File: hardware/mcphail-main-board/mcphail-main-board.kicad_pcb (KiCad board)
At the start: 2 copper layers, 80.6 x 56.6 mm, 143 parts, among them J1 INSECT DETECTION, J2 EMITTERS, J3 BREAKOUT, J4 MICRO SD, J5 MICRO USB, J6 PROG/BOOT, J7 FONA 808, J8 INPUT 6V-9V, J9 JST PH, U1 MCP6004, U10 BUCK-BOOST 5V TPS63060, U11 MCP1703, U2 MCP6004, U3 TLV274, U4 MCP6001, U5 ADS1118, U6 ATSAMD21G18A, U7 24AA1025 EEPROM, U8 MCP7940N RTC, U9 MCP73871, X1 16MHz, X2 32.768kHz

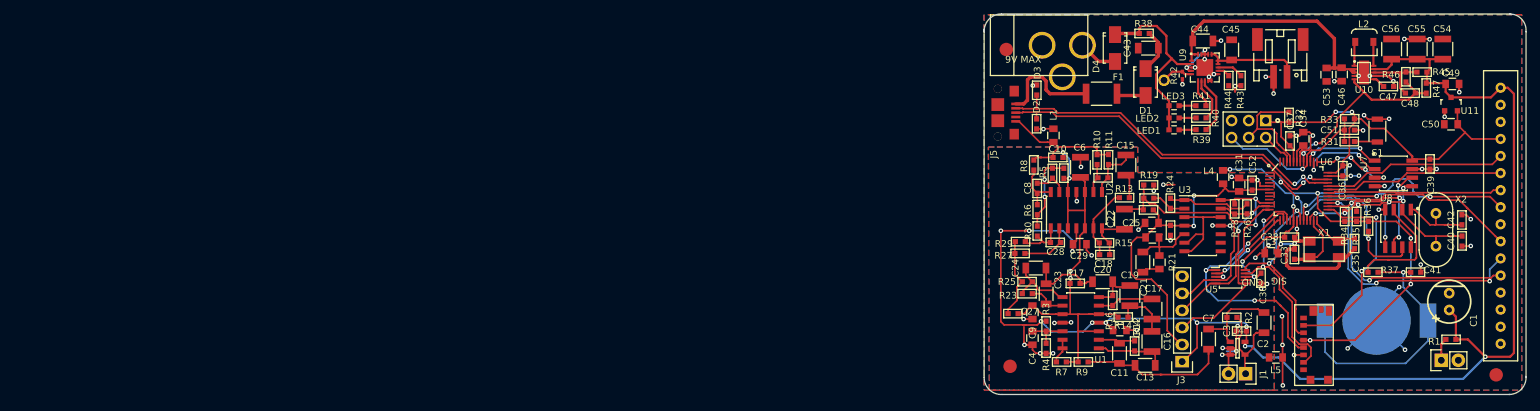
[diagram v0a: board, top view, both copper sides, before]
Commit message: Release v1.0 McPhail Main Board
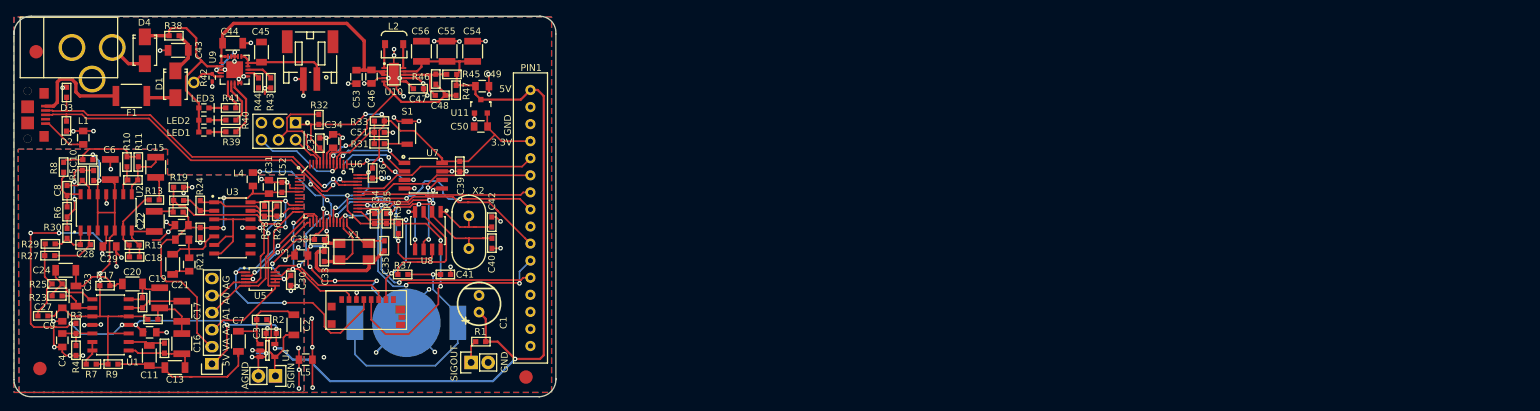
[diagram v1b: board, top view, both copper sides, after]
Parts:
- moved BAT1 144.4 mm to (81.7, 87.8)
- moved C1 144.4 mm to (92.5, 84.9)
- moved C10 144.4 mm to (34.3, 63.5)
- moved C11 144.4 mm to (43.4, 92.6)
- moved C12 144.4 mm to (40.9, 66.5)
- moved C13 144.4 mm to (47.2, 94.4)
- moved C14 144.4 mm to (43.5, 89.2)
- moved C15 144.4 mm to (44.4, 64.6)
- moved C16 144.4 mm to (48.2, 90.9)
- moved C17 144.4 mm to (48.2, 86.0)
- moved C2 144.4 mm to (64.9, 88.1)
- moved C20 144.4 mm to (40.9, 82.0)
- moved C21 144.4 mm to (46.9, 79.1)
- moved C22 144.4 mm to (44.1, 72.7)
- moved C23 144.4 mm to (32.5, 83.8)
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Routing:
- net GND: track 127.3 -> 171.4 mm, vias 45 -> 57
- net AGND: track 52.7 -> 67.3 mm, vias 26 -> 32
- net /Microcontroller/D7_CS: track 30.8 -> 21.0 mm
- net /Microcontroller/MISO: track 34.3 -> 25.8 mm
- net +3V3: track 156.4 -> 150.2 mm, vias 11 -> 10
- net /Microcontroller/SCLK: track 40.6 -> 45.8 mm
- net /Microcontroller/MOSI: track 28.4 -> 30.1 mm
- net (no net): track 1.71 -> 0.00 mm
- net /Microcontroller/SDA: track 28.5 -> 29.2 mm
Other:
- board text added: "3.3V"
- board text added: "5V"
- board text added: "5V VA A2 A1 A0 AG"
- board text added: "AGND"
- board text added: "FABRICATION NOTES 1. THIS IS A 2 LAYER BOARD. 2. EXTERNAL LAYERS SHALL HAVE 1 OZ COPPER. 3. MATERIAL: FR4 AND 0.062 INCH +/- 10% THICK. 4. BOARDS SHALL BE ROHS COMPLIANT. 5. MANUFACTURE IN ACCORDANCE WITH IPC-6012 CLASS 2 6. MASK: BOTH SIDES OF THE BOARD SHALL HAVE SOLDER MASK (ANY COLOR) OVER BARE COPPER. 7. SILK: BOTH SIDES OF THE BOARD SHALL HAVE WHITE SILKSCREEN. DO NOT PLACE SILK OVER BARE C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"
- board text added: "McPhail Trap Main Board v1.0 Kyle Birchard and Jenner Hanni jenner@wickerbox.net"
- board text added: "PIN1"
- board text added: "SIGIN"
- board text added: "SIGOUT"
- board text removed: "9V MAX"
- board text removed: "SIG"
